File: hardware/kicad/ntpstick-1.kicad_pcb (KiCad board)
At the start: 2 copper layers, 140 x 25 mm, 78 parts, among them CON1 PDI, IC1 W5500, IC2 ATXMEGA128A4-A, IC3 24AA02E48, J1 MOUNT0, J2 MOUNT1, P1 EIA 568B, P2 CONN_01X05, U1 TG110-E*N5_N5, U2 LM2672, U3 UBLOX-GPS, U4 MAX5805BAUB+, X1 25MHz, X2 VCXO-7x5

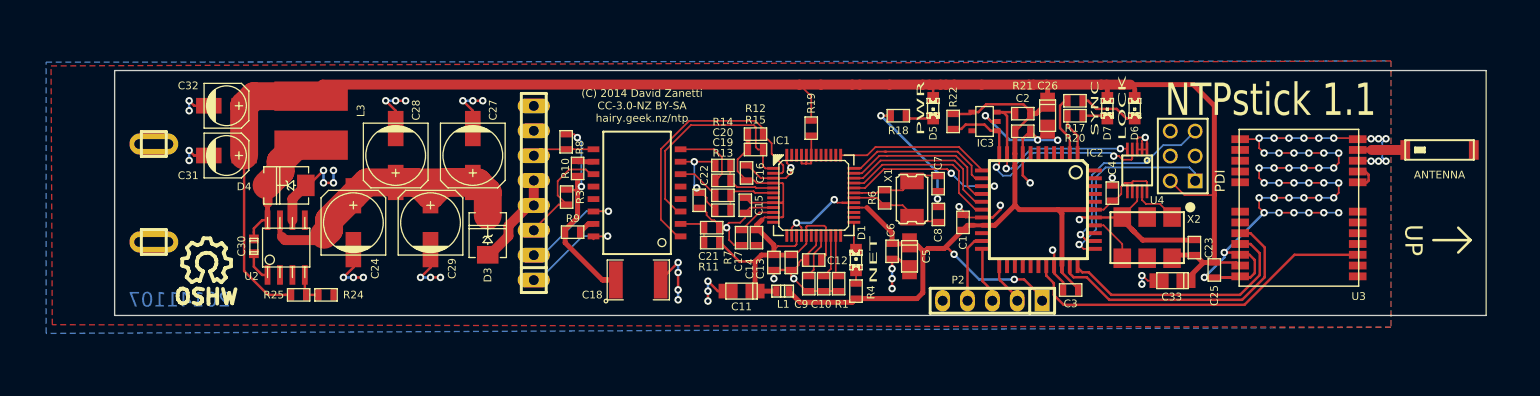
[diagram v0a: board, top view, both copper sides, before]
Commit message: Version 1.2 HW design
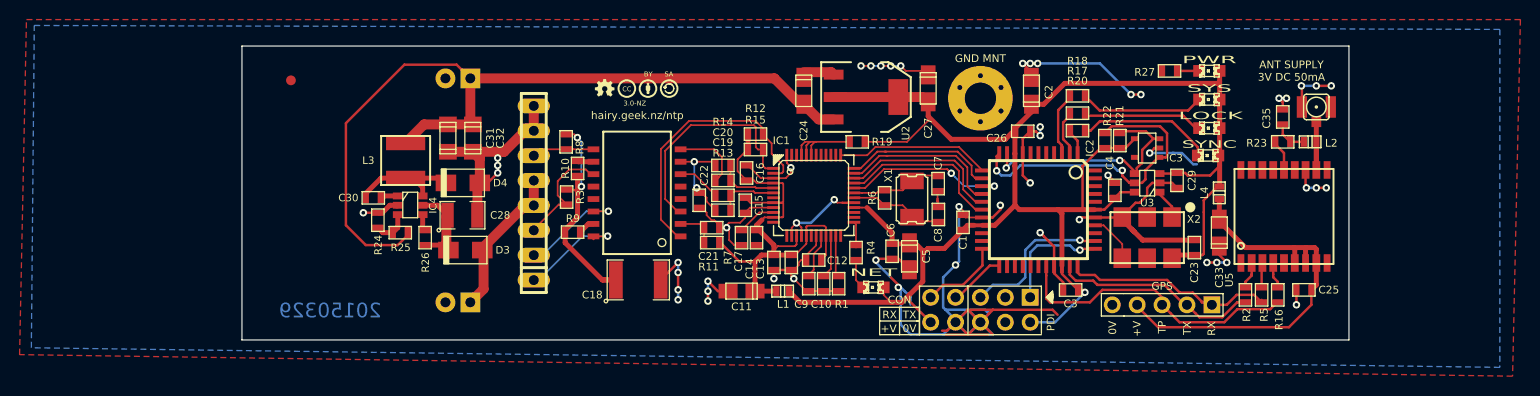
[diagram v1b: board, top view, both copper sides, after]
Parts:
- removed CON1: PDI, pin_array_3x2
- removed SYM: Symbol_OSHW-Logo_SilkScreen_07Jul2012, Symbols:Symbol_OSHW-Logo_SilkScreen
- removed U4: MAX5805BAUB+, SMD_Packages:MSOP10-0.5
- added C35: 100nF, SMD_Packages:SM0603, F.Cu at (150.2, 54.7)
- added D2: PWR, LEDs:LED-0805, F.Cu at (142.7, 50.0)
- added FIDUCIAL: val**, Freetronics Footprints:FIDUCIAL, F.Cu at (49.0, 51.0)
- added IC4: LMR16006, SMD_Packages:SOT23_6, F.Cu at (61.2, 63.8)
- added J3: MOUNT2, 4-40-HOLE, F.Cu at (119.4, 52.8)
- added L2: 27nH, Walter Inductors:inductor_smd_0603, F.Cu at (153.0, 57.3)
- added L4: 250mA, Walter Inductors:inductor_smd_0603, F.Cu at (143.8, 62.5)
- added LOGO_CC: VAL**, Freetronics Footprints:LOGO_CC_1.9mm, F.Cu at (83.3, 51.8)
- added LOGO_CC_BY: VAL**, CC logos:LOGO_CC_BY_1.9mm, F.Cu at (85.4, 51.8)
- added LOGO_CC_SA: VAL**, LOGO_CC_SA_1.9mm, F.Cu at (87.6, 51.8)
- added LOGO_OSHW_silkscreen_2mm: val**, Freetronics Footprints:LOGO_OSHW_silkscreen_2mm, F.Cu at (81.0, 51.8)
- added P3: PDI-SER, Pin_Headers:Pin_Header_Straight_2x05, F.Cu at (119.4, 74.4)
- added P7: 5V, Pin_Headers:Pin_Header_Straight_1x02, F.Cu at (66.0, 50.8)
- added P8: VIN, Pin_Headers:Pin_Header_Straight_1x02, F.Cu at (66.0, 73.7)
- added R16: 1k, SMD_Packages:SM0603, F.Cu at (149.7, 72.9)
- added R2: 1k, SMD_Packages:SM0603, F.Cu at (146.4, 72.9)
- added R23: 10, SMD_Packages:SM0603, F.Cu at (150.2, 57.3)
- added R26: 100k, SMD_Packages:SM0603, F.Cu at (62.7, 67.1)
- added R27: 1k, SMD_Packages:SM0603, F.Cu at (138.7, 50.0)
- added R5: 1k, SMD_Packages:SM0603, F.Cu at (148.1, 72.9)
- added SERIAL_LABEL: VAL**, Dymo 12x24:SERIAL_LABEL, B.Cu at (85.9, 62.7)
- added U5: UBLOX-MAX, UBLOX MAX:UBLOX-MAX-8-POLY, F.Cu at (150.4, 64.9)
- ANT1: value ANTENNA -> ANTENNA_SHIELD; footprint 1575AT43A0-JOHANSON -> Walter RF Conn:coaxial_u.fl-r-smt-1
- C24, C27: value 22uF -> 10uF; footprint Capacitors_SMD:c_elec_6.3x5.8 -> Water SMD Cap:c_tant_A
- C25: footprint SM0603 -> SMD_Packages:SM0603
- C28: value 22uF -> 3.3uF; footprint Capacitors_SMD:c_elec_6.3x5.8 -> SMD_Packages:SM1210
- C29: value 22uF -> 100nF; footprint Capacitors_SMD:c_elec_6.3x5.8 -> SMD_Packages:SM0603
- C30: value 10nF -> 100nF; footprint Capacitors_SMD:c_0603 -> SMD_Packages:SM0603
- C31, C32: value 22uF -> 10uF; footprint Capacitors_SMD:c_elec_4x5.3 -> Water SMD Cap:c_1206
- C33: footprint c_tant_A -> Water SMD Cap:c_tant_A
- D3: footprint DO-214AA(SMB) -> Walter Diodes:do214ac
- D4: footprint SMD_Packages:DO-214AA(SMB) -> Walter Diodes:do214ac
- D5: value PWR -> SYS
- L3: value 47uH -> 6.8uH; footprint Walter Inductors:inductor_smd_8x5mm -> Bourns Inductor:inductor_bourns_srn5040
- P2: value CONN_01X05 -> GPS; footprint Walter Pin Headers:pin_strip_5 -> Pin_Headers:Pin_Header_Straight_1x05
- R24: value NP -> 6.49k
- R25: value 0 -> 36.0k
- U2: value LM2672 -> NCP1117ST33T3G; footprint Walter SMD DIL:so-8 -> SMD_Packages:SOT223
- U3: value UBLOX-GPS -> MCP4725AxT-E/CH; footprint UBLOX-GPS -> SMD_Packages:SOT23_6
- moved C29 76.3 mm to (139.4, 61.2)
- moved U2 61.1 mm to (107.7, 52.7), turned to 270 degrees
- moved C24 47.9 mm to (101.3, 52.1)
- moved C27 47.0 mm to (114.0, 51.8), turned to 90 degrees
- moved D5 28.2 mm to (142.7, 53.0), turned to 180 degrees
- moved C32 25.4 mm to (67.6, 56.9), turned to 90 degrees
- moved C31 22.7 mm to (65.0, 56.9), turned to 90 degrees
- moved R18 18.4 mm to (129.3, 52.6)
- moved D4 18.0 mm to (66.5, 61.5)
- moved P2 17.3 mm to (137.9, 73.9)
- moved IC3 16.8 mm to (136.4, 57.9)
- moved U3 15.7 mm to (136.4, 61.5), turned to 90 degrees
- moved R22 15.6 mm to (132.1, 57.1), turned to 270 degrees
- moved ANT1 13.3 mm to (153.7, 53.7)
- moved C30 13.2 mm to (57.4, 63.0), turned to 0 degrees
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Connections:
- net /NTP Stick Ethernet/RXN renamed /NTP Stick Ethernet/RX_N
- net /NTP Stick Ethernet/RXP renamed /NTP Stick Ethernet/RX_P
- net /NTP Stick Ethernet/TXN renamed /NTP Stick Ethernet/TX_N
- net /NTP Stick Ethernet/TXP renamed /NTP Stick Ethernet/TX_P
- net Net-(C19-Pad2) renamed /NTP Stick Ethernet/RX1_P
- net Net-(C20-Pad2) renamed /NTP Stick Ethernet/RX1_N
- ANT1 pad 2: (no net) -> GND
- C24 pad 1: Net-(C24-Pad1) -> +5V
- C25 pad 1: +3.3V -> /NTP Stick System/GPS_VCC
- C27 pad 1: Net-(C24-Pad1) -> +3.3V
- C28 pad 1: Net-(C24-Pad1) -> Net-(C28-Pad1)
- C29 pad 1: Net-(C24-Pad1) -> GND
- C29 pad 2: GND -> +3.3V
- C31 pad 1: +3.3V -> +5V
- C32 pad 1: +3.3V -> +5V
- C33 pad 1: +3.3V -> /NTP Stick System/GPS_VCC
- D1 pad 1: Net-(D1-Pad1) -> +3.3V
- D1 pad 2: /NTP Stick Ethernet/LNKLED -> Net-(D1-Pad2)
- D3 pad 2: Net-(C24-Pad1) -> Net-(C28-Pad1)
- D4 pad 2: Net-(C30-Pad2) -> Net-(C30-Pad1)
- IC2 pad 21: /NTP Stick System/FACRSTn -> Net-(IC2-Pad21)
- IC2 pad 29: /NTP Stick System/GPS_TIMEPULSE -> /NTP Stick System/GPS_TP
- IC2 pad 3: Net-(IC2-Pad3) -> /NTP Stick System/LED_PWR
- IC2 pad 32: /NTP Stick System/GPS_TX -> /NTP Stick System/GPS_TXD
- IC2 pad 33: /NTP Stick System/GPS_RX -> /NTP Stick System/GPS_RXD
- L3 pad 1: Net-(C30-Pad2) -> Net-(C30-Pad1)
- L3 pad 2: +3.3V -> +5V
- P2 pad 1: +3.3V -> /NTP Stick System/GPS_RXD
- P2 pad 2: /NTP Stick System/CON_TX -> /NTP Stick System/GPS_TXD
- P2 pad 3: /NTP Stick System/CON_RX -> /NTP Stick System/GPS_TP
- P2 pad 4: /NTP Stick System/FACRSTn -> /NTP Stick System/GPS_VCC
- R18 pad 1: GND -> /NTP Stick System/LED_PWR
- R24 pad 2: Net-(R24-Pad2) -> Net-(IC4-Pad3)
- R25 pad 1: Net-(R24-Pad2) -> Net-(IC4-Pad3)
- R25 pad 2: +3.3V -> +5V
- R4 pad 1: Net-(D1-Pad1) -> /NTP Stick Ethernet/LNKLED
- R4 pad 2: +3.3V -> Net-(D1-Pad2)
- U2 pad 1: Net-(C30-Pad1) -> GND
- U2 pad 2: Net-(U2-Pad2) -> +3.3V
- U2 pad 3: Net-(U2-Pad3) -> +5V
- U3 pad 1: Net-(U3-Pad1) -> /NTP Stick System/OSC_CTRL
- U3 pad 2: Net-(U3-Pad2) -> GND
- U3 pad 3: /NTP Stick System/GPS_TIMEPULSE -> +3.3V
- U3 pad 4: Net-(U3-Pad4) -> /NTP Stick System/SDA
- U3 pad 5: Net-(U3-Pad5) -> /NTP Stick System/SCL
- U3 pad 6: Net-(U3-Pad6) -> +3.3V
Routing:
- net +3.3V: track 272.7 -> 180.7 mm, vias 2 -> 1
- net +5V: track 0.00 -> 86.0 mm
- net Net-(C24-Pad1): track 49.6 -> 0.00 mm
- net /NTP Stick System/GPS_VCC: track 0.00 -> 42.2 mm
- net /NTP Stick System/GPS_TIMEPULSE: track 37.0 -> 0.00 mm
- net /NTP Stick System/GPS_TP: track 0.00 -> 30.4 mm
- net /NTP Stick System/GPS_TX: track 29.0 -> 2.75 mm
- net /NTP Stick System/GPS_RX: track 25.6 -> 2.52 mm
- net /NTP Stick System/GPS_RXD: track 0.00 -> 22.2 mm
- net /NTP Stick System/GPS_TXD: track 0.00 -> 21.3 mm
- net Net-(C30-Pad2): track 14.4 -> 1.91 mm
- net Net-(D7-Pad2): track 2.66 -> 13.9 mm
- net Net-(C30-Pad1): track 3.07 -> 13.2 mm
- net Net-(D5-Pad2): track 2.91 -> 12.7 mm
- net Net-(C28-Pad1): track 0.00 -> 9.33 mm
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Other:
- board size 140 x 25 mm -> 113 x 30 mm
- board text added: "+V"
- board text added: "0V"
- board text added: "20150329"
- board text added: "3.0-NZ"
- board text added: "ANT SUPPLY 3V DC 50mA"
- board text added: "BY"
- board text added: "CON"
- board text added: "GND MNT"
- board text added: "GPS"
- board text added: "NTPstick 1.2"
- board text added: "PDI"
- board text added: "RX"
- board text added: "SA"
- board text added: "TIA/EIA-568B +V BLU/BLUW GND BRN/BRNW"
- board text added: "TP"
- board text added: "TX"
- board text added: "hairy.geek.nz/ntp"
- board text removed: "(C) 2014 David Zanetti CC-3.0-NZ BY-SA hairy.geek.nz/ntp"
- board text removed: "20141107"
- board text removed: "NTPstick 1.1"
- board text removed: "RESET"
- board text removed: "TIA/EIA-568B DC 7-36V +V BLU/BLUW GND BRN/BRNW"
- board text removed: "UP"
